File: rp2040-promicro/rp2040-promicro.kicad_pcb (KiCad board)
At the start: 2 copper layers, 17.9 x 39.8 mm, 30 parts, among them J2 ProMicro-LeftPin, J3 ProMicro-RightPin, P1 USB2.0_C_12pin, SW1 SW_Push, U1 RP2040, U2 W25Q128JVS, U3 AZ1117-3.3, Y1 Crystal_GND24

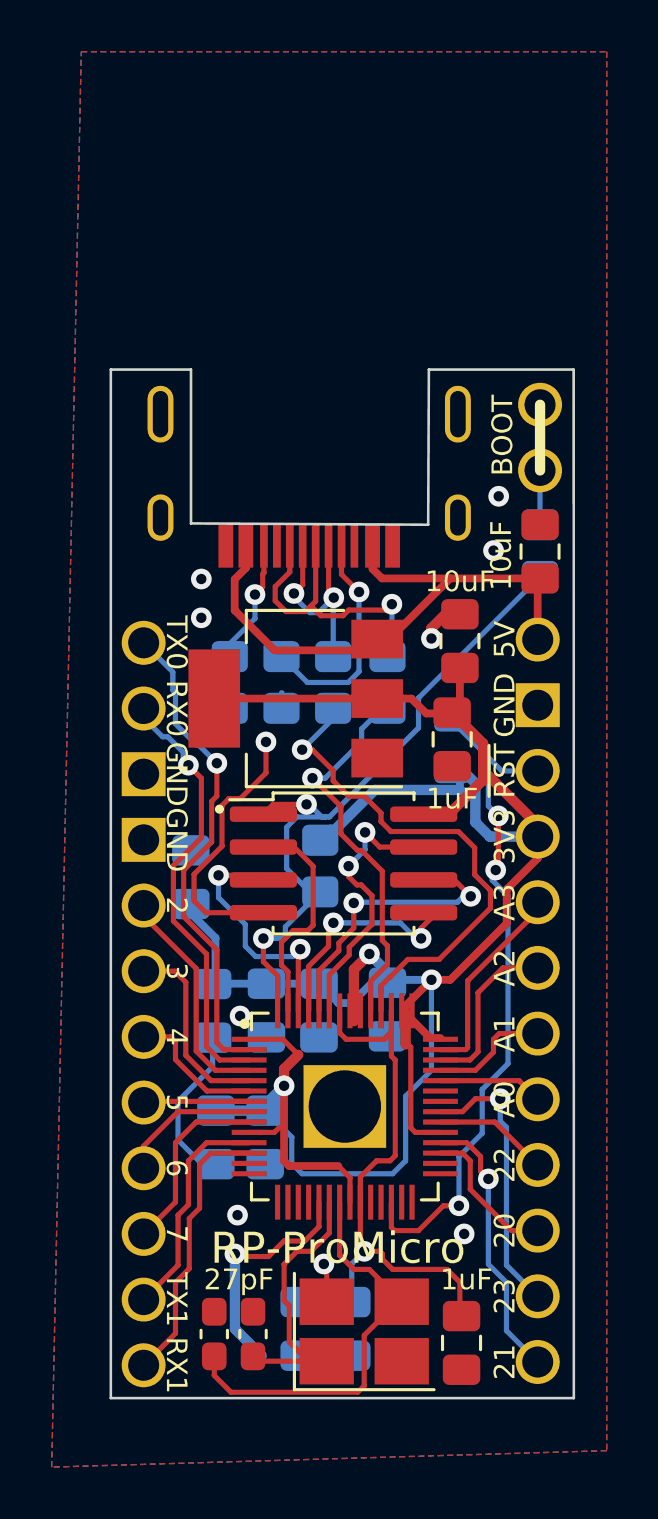
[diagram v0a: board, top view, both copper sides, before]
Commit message: promicro v2
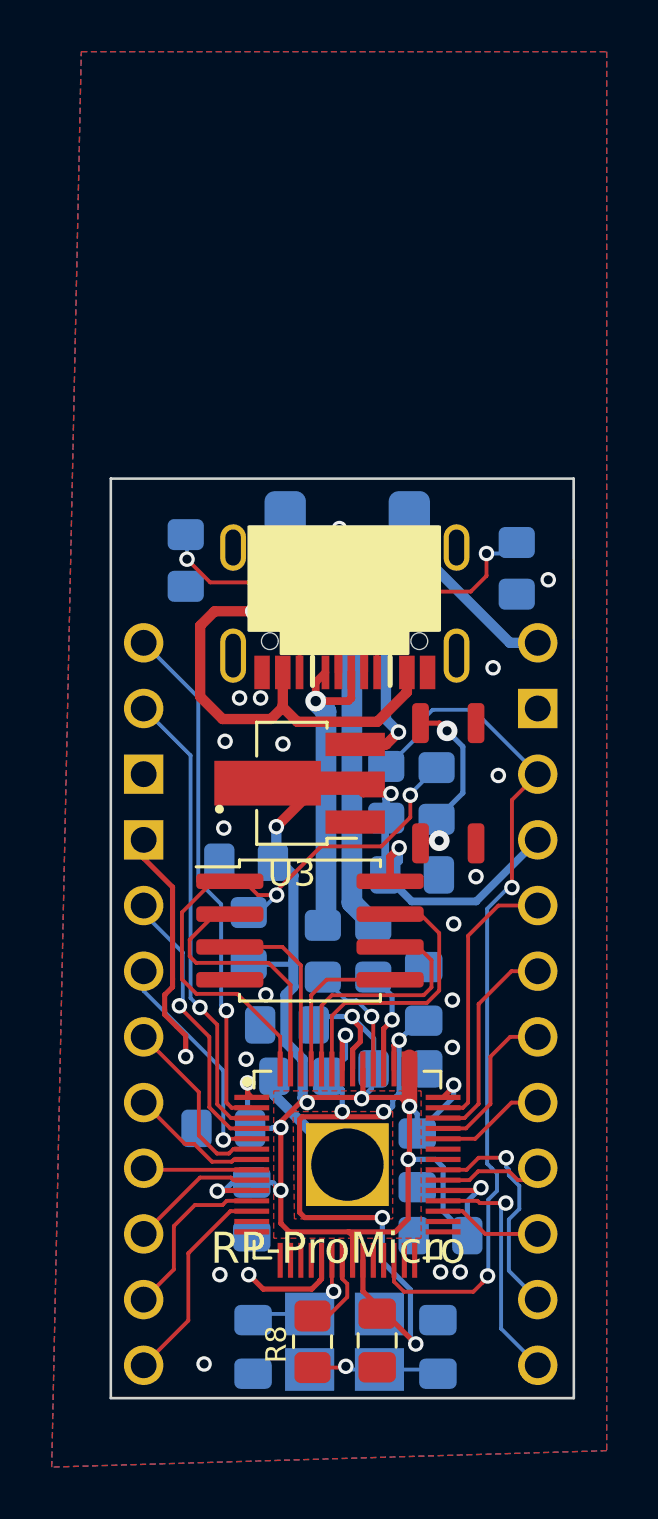
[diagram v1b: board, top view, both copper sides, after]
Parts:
- removed C4: 100nF, rp2040-dev-board:Capacitor_0805_2012
- removed P1: USB2.0_C_12pin, rp2040-dev-board:USB-C-12-Pin-MidMount-ali-v2
- added F1: Polyfuse, $74th:ResettableFuse_KT6-1100SMDI, B.Cu at (59.1, 47.0)
- added J1: USB2.0_C_v3, $74th:USB-C-12-Pin-SMD, F.Cu at (59.0, 47.6)
- added R8: 1kR, rp2040-dev-board:Register_0805_2012, F.Cu at (57.9, 78.4)
- C11, C12: footprint rp2040-dev-board:Capacitor_0603_1608 -> rp2040-dev-board:Capacitor_0805_2012; moved to B.Cu
- C14, C15, C3, C5: moved to B.Cu
- C2: moved to F.Cu
- J2: footprint rp2040-dev-board:LeftPin -> $74th:ProMicro_LIKE_LEFT
- J3: footprint rp2040-dev-board:RightPin -> $74th:ProMicro_LIKE_RIGHT
- SW1: footprint rp2040-dev-board:BOOT -> rp2040-dev-board:SKRPABE010
- U3: footprint rp2040-dev-board:Regulator-AMS1117-SOT-223 -> $74th:Regulator_AMS1117_SOT-89
- Y1: footprint Crystal:Crystal_SMD_3225-4Pin_3.2x2.5mm_HandSoldering -> rp2040-dev-board:Crystal_SMD_3225-4Pin_3.2x2.5mm_HandSoldering; moved to B.Cu
- moved J3 15.4 mm to (66.5, 66.5)
- moved J2 14.0 mm to (51.3, 65.2)
- moved C3 13.6 mm to (62.1, 64.8), turned to 90 degrees
- moved C5 12.8 mm to (56.8, 66.0), turned to 180 degrees
- moved SW1 12.6 mm to (63.0, 56.7), turned to -90 degrees
- moved C15 11.9 mm to (55.2, 59.8), turned to 180 degrees
- moved C9 11.0 mm to (61.2, 67.7), turned to 0 degrees
- moved R1 10.7 mm to (58.3, 63.1)
- moved R2 10.5 mm to (60.2, 63.1)
- moved R5 10.1 mm to (65.6, 48.5)
- moved C1 9.96 mm to (57.4, 68.0), turned to 180 degrees
- moved R3 9.95 mm to (62.7, 57.0), turned to 90 degrees
- moved C10 8.98 mm to (62.8, 74.2), turned to 180 degrees
- moved C12 8.67 mm to (62.6, 78.5)
- moved C8 8.22 mm to (61.9, 71.3)
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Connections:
- C12 pad 2: XOUT -> Net-(C12-Pad2)
- J2 pad 1: 9/RX1 -> 0/TX0
- J2 pad 10: GND -> 7
- J2 pad 11: 1/RX0 -> 8/TX1
- J2 pad 12: 0/TX0 -> 9/RX1
- J2 pad 2: 8/TX1 -> 1/RX0
- J2 pad 3: 7 -> GND
- J2 pad 4: 6 -> GND
- J2 pad 5: 5 -> 2
- J2 pad 6: 4 -> 3
- J2 pad 7: 3 -> 4
- J2 pad 8: 2 -> 5
- J2 pad 9: GND -> 6
- J3 pad 1: +5V -> 21
- J3 pad 10: 20 -> ~{RESET}
- J3 pad 11: 23 -> GND
- J3 pad 12: 21 -> +5V
- J3 pad 2: GND -> 23
- J3 pad 3: ~{RESET} -> 20
- J3 pad 4: +3V3 -> 22
- J3 pad 5: A3 -> A0
- J3 pad 6: A2 -> A1
- J3 pad 7: A1 -> A2
- J3 pad 8: A0 -> A3
- J3 pad 9: 22 -> +3V3
- Y1 pad 3: XOUT -> Net-(C12-Pad2)
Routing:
- net Net-(F1-Pad1): track 0.00 -> 19.9 mm, vias 0 -> 1
- net Net-(R2-Pad1): track 19.8 -> 3.99 mm
- net XOUT: track 16.0 -> 3.15 mm
- net +3V3: track 95.6 -> 83.1 mm, vias 3 -> 14
- net GND: track 29.6 -> 17.9 mm, vias 11 -> 22
- net Net-(R1-Pad1): track 14.7 -> 4.60 mm
- net +1V1: track 22.7 -> 30.5 mm, vias 1 -> 6
- net ~{RESET}: track 26.9 -> 33.7 mm, vias 3 -> 2
- net USB_DM: track 8.45 -> 14.6 mm, vias 2 -> 1
- net XIN: track 10.5 -> 4.81 mm, vias 0 -> 1
- net +5V: track 22.7 -> 17.1 mm, vias 0 -> 1
- net Net-(C12-Pad2): track 0.00 -> 4.99 mm, vias 0 -> 1
- net Net-(R3-Pad1): track 2.10 -> 6.89 mm, vias 0 -> 2
- net Net-(J1-Pad6): track 4.81 -> 8.71 mm
- net QSPI_SS: track 26.9 -> 23.1 mm
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- added copper zone on F.Cu, net +1V1
- added copper zone on F.Cu, net +3V3
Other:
- board size 17.9 x 39.8 mm -> 17.9 x 35.6 mm
- board text added: "RP-ProMicro v2.0.0"
- board text removed: "RP-ProMicro v1.0.1"
